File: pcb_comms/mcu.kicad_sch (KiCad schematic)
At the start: 25 parts, among them U2 STM32WLE5CCU6, Y1 G43270018, Y3 32MHz

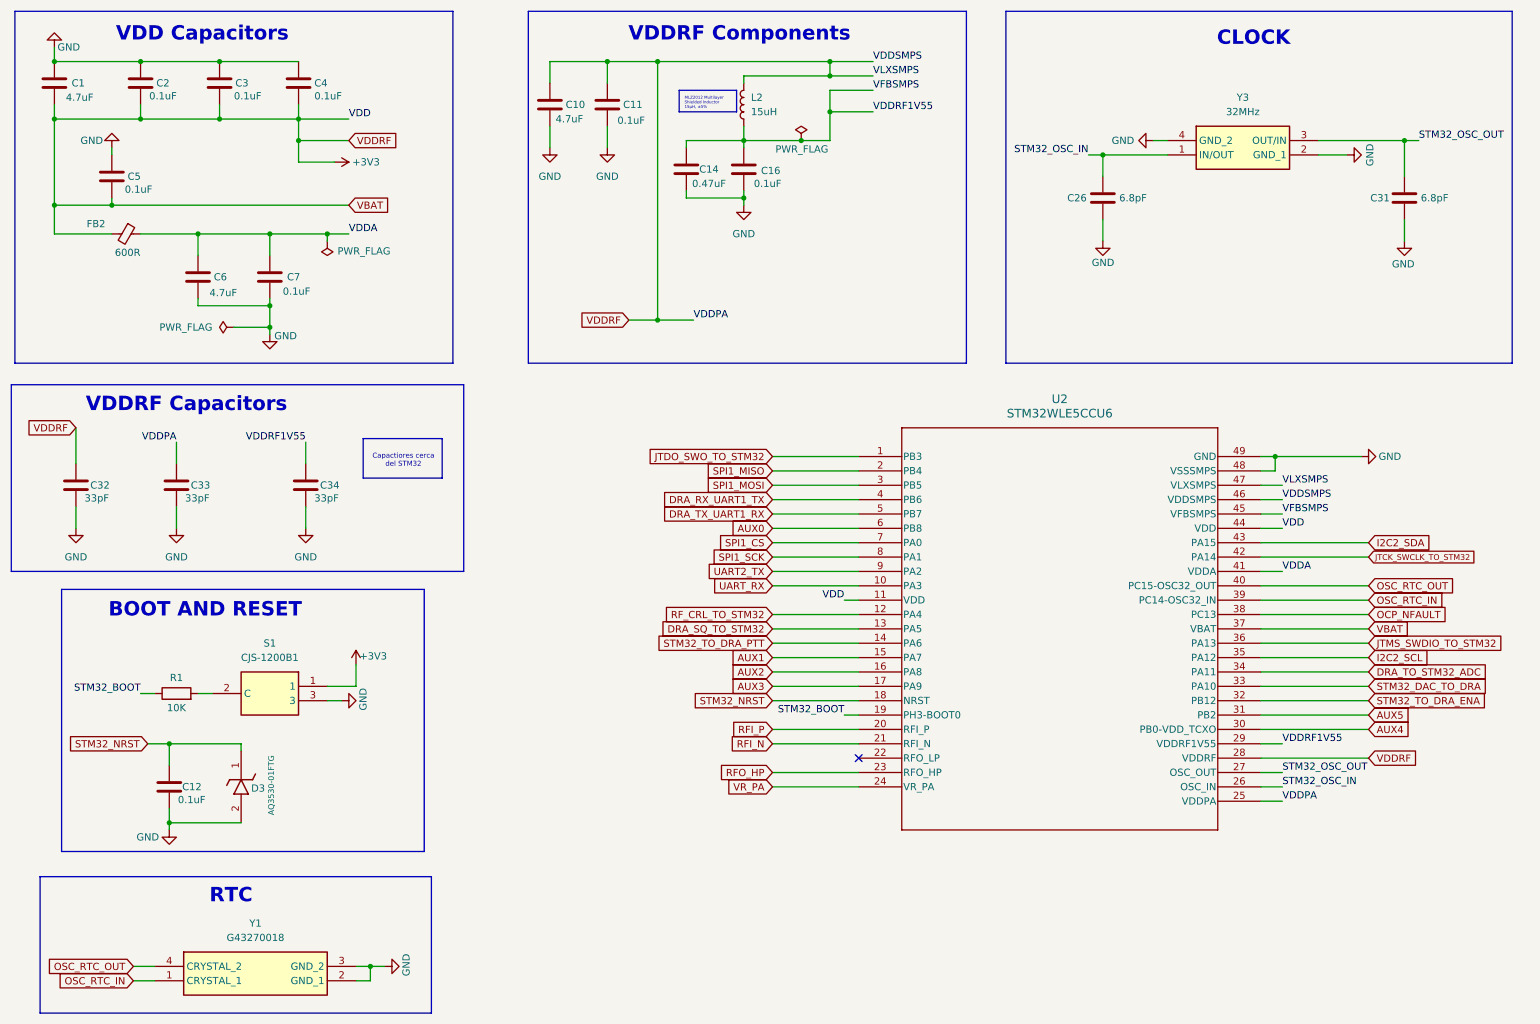
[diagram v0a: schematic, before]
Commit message: Route pcb
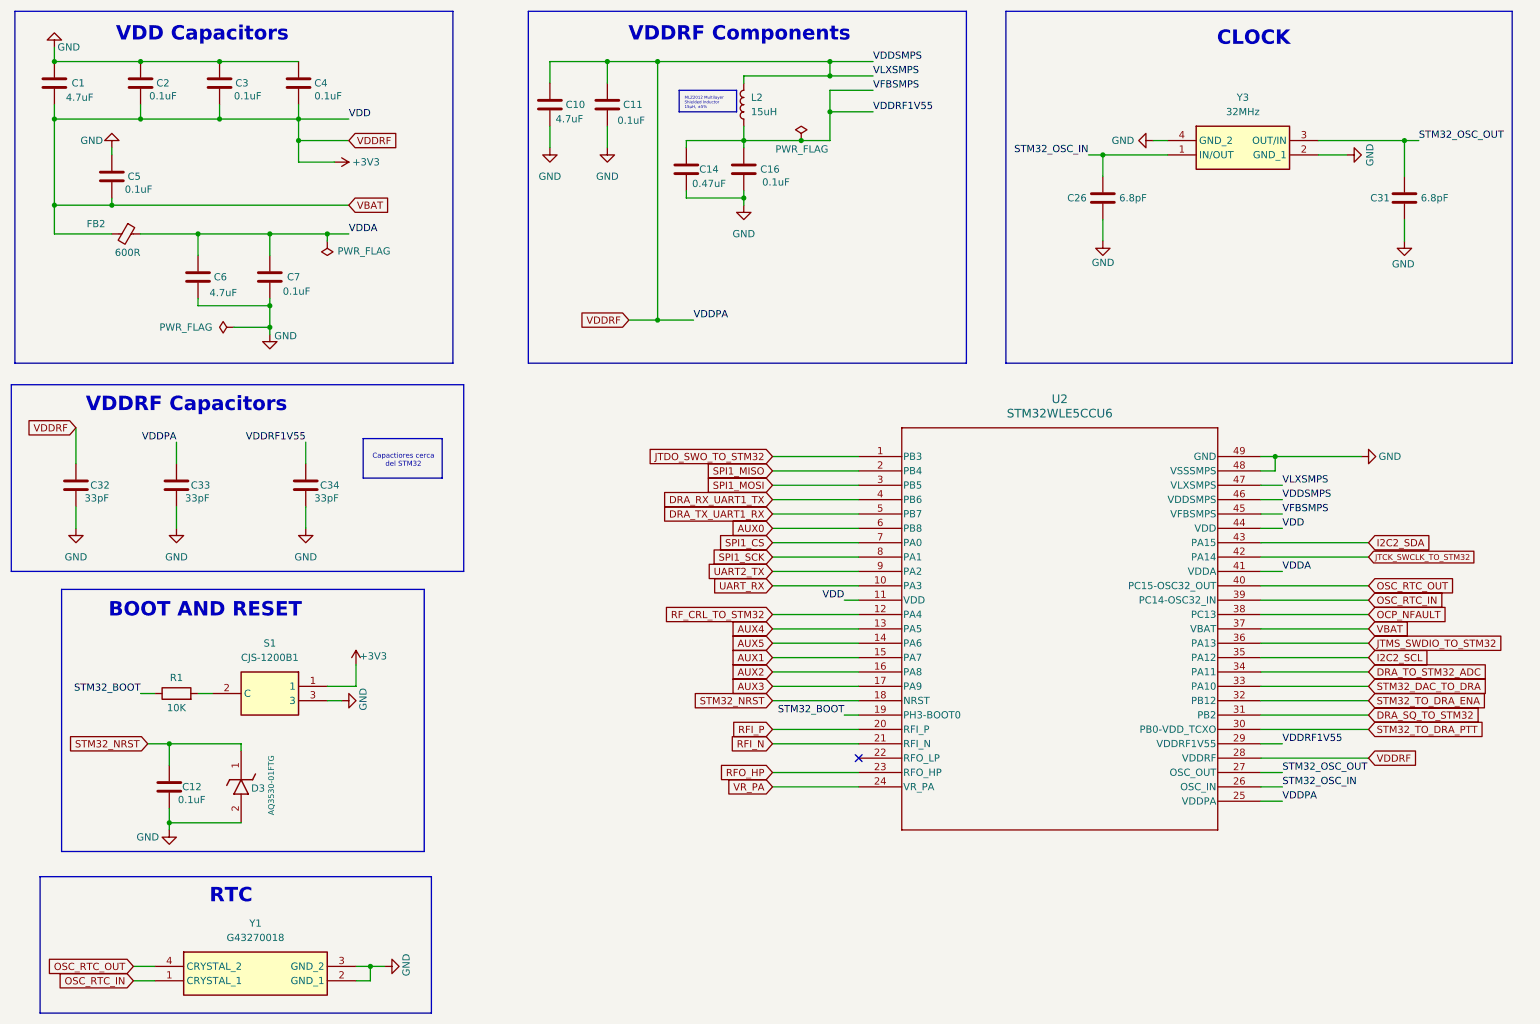
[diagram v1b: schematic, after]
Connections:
- net AUX4: now also U2.13 (PA5); no longer U2.30 (PB0-VDD_TCXO)
- net AUX5: now also U2.14 (PA6); no longer U2.31 (PB2)
- net DRA_SQ_TO_STM32: now also U2.31 (PB2); no longer U2.13 (PA5)
- net STM32_TO_DRA_PTT: now also U2.30 (PB0-VDD_TCXO); no longer U2.14 (PA6)
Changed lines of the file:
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@@
 	(wire
 		(pts
+			(xy 152.4 129.54) (xy 167.64 129.54)
+		)
+		(stroke
+			(width 0)
+			(type default)
+		)
+	)
+	(wire
+		(pts
 			(xy 147.32 40.64) (xy 147.32 41.91)
 		)
@@
 	(wire
 		(pts
-			(xy 152.4 127) (xy 167.64 127)
-		)
-		(stroke
-			(width 0)
-			(type default)
-		)
-	)
-	(wire
-		(pts
 			(xy 241.3 99.06) (xy 241.3 96.52)
 		)
@@
 	(wire
 		(pts
+			(xy 152.4 127) (xy 167.64 127)
+		)
+		(stroke
+			(width 0)
+			(type default)
+		)
+	)
+	(wire
+		(pts
 			(xy 152.4 134.62) (xy 167.64 134.62)
 		)
@@
 	(wire
 		(pts
-			(xy 238.76 142.24) (xy 257.81 142.24)
-		)
-		(stroke
-			(width 0)
-			(type default)
-		)
-	)
-	(wire
-		(pts
 			(xy 25.4 57.15) (xy 35.56 57.15)
 		)
@@
 	(wire
 		(pts
-			(xy 238.76 144.78) (xy 257.81 144.78)
-		)
-		(stroke
-			(width 0)
-			(type default)
-		)
-	)
-	(wire
-		(pts
 			(xy 45.72 147.32) (xy 58.42 147.32)
 		)
@@
 	(wire
 		(pts
+			(xy 238.76 142.24) (xy 257.81 142.24)
+		)
+		(stroke
+			(width 0)
+			(type default)
+		)
+	)
+	(wire
+		(pts
 			(xy 165.1 121.92) (xy 167.64 121.92)
 		)
@@
 	(wire
 		(pts
-			(xy 39.37 186.69) (xy 43.18 186.69)
+			(xy 238.76 144.78) (xy 257.81 144.78)
 		)
 		(stroke
@@
 	(wire
 		(pts
-			(xy 77.47 40.64) (xy 68.58 40.64)
+			(xy 39.37 186.69) (xy 43.18 186.69)
 		)
 		(stroke
@@
 	(wire
 		(pts
-			(xy 73.66 57.15) (xy 73.66 58.42)
+			(xy 77.47 40.64) (xy 68.58 40.64)
 		)
 		(stroke
@@
 	(wire
 		(pts
-			(xy 113.03 26.67) (xy 113.03 30.48)
+			(xy 73.66 57.15) (xy 73.66 58.42)
 		)
 		(stroke
@@
 	(wire
 		(pts
-			(xy 152.4 139.7) (xy 167.64 139.7)
+			(xy 113.03 26.67) (xy 113.03 30.48)
 		)
 		(stroke
@@
 	(wire
 		(pts
-			(xy 78.74 137.16) (xy 78.74 133.35)
+			(xy 152.4 139.7) (xy 167.64 139.7)
 		)
 		(stroke
@@
 	(wire
 		(pts
-			(xy 152.4 129.54) (xy 167.64 129.54)
+			(xy 78.74 137.16) (xy 78.74 133.35)
 		)
 		(stroke
@@
 	(global_label "DRA_SQ_TO_STM32"
 		(shape input)
-		(at 152.4 127 180)
+		(at 257.81 142.24 0)
 		(effects
 			(font
 				(size 1.27 1.27)
 			)
-			(justify right)
+			(justify left)
 		)
 		(property "Intersheetrefs" "${INTERSHEET_REFS}"
-			(at 130.7278 114.3 0)
+			(at 279.4822 129.54 0)
 			(effects
 				(font
 					(size 1.27 1.27)
 				)
-				(justify right)
+				(justify left)
 				(hide yes)
 			)
@@
 	(global_label "STM32_TO_DRA_PTT"
 		(shape input)
-		(at 152.4 129.54 180)
+		(at 257.81 144.78 0)
 		(fields_autoplaced yes)
 		(effects
@@
 				(size 1.27 1.27)
 			)
-			(justify right)
+			(justify left)
 		)
 		(property "Intersheetrefs" "${INTERSHEET_REFS}"
-			(at 131.3326 129.54 0)
+			(at 278.8774 144.78 0)
 			(effects
 				(font
 					(size 1.27 1.27)
 				)
-				(justify right)
+				(justify left)
 				(hide yes)
 			)
@@
 	(global_label "AUX4"
 		(shape input)
-		(at 257.81 144.78 0)
+		(at 152.4 127 180)
 		(fields_autoplaced yes)
 		(effects
@@
 				(size 1.27 1.27)
 			)
-			(justify left)
+			(justify right)
 		)
 		(property "Intersheetrefs" "${INTERSHEET_REFS}"
-			(at 265.6333 144.78 0)
+			(at 144.5767 127 0)
 			(effects
 				(font
 					(size 1.27 1.27)
 				)
-				(justify left)
+				(justify right)
 				(hide yes)
 			)
@@
 	(global_label "AUX5"
 		(shape input)
-		(at 257.81 142.24 0)
+		(at 152.4 129.54 180)
 		(fields_autoplaced yes)
 		(effects
@@
 				(size 1.27 1.27)
 			)
-			(justify left)
+			(justify right)
 		)
 		(property "Intersheetrefs" "${INTERSHEET_REFS}"
-			(at 265.6333 142.24 0)
+			(at 144.5767 129.54 0)
 			(effects
 				(font
 					(size 1.27 1.27)
 				)
-				(justify left)
+				(justify right)
 				(hide yes)
 			)
@@
 		(lib_id "Device:C")
 		(at 147.32 45.72 0)
+		(mirror y)
 		(unit 1)
 		(exclude_from_sim no)
@@
 		(dnp no)
 		(property "Reference" "C16"
-			(at 150.368 45.974 0)
+			(at 153.67 45.72 0)
 			(effects
 				(font
@@
 		)
 		(property "Value" "0.1uF"
-			(at 149.098 48.26 0)
+			(at 155.448 48.006 0)
 			(effects
 				(font
@@
 		)
 		(property "Footprint" "Capacitor_SMD:C_0805_2012Metric_Pad1.18x1.45mm_HandSolder"
-			(at 148.2852 49.53 0)
+			(at 146.3548 49.53 0)
 			(effects
 				(font
@@
 		(on_board yes)
 		(dnp no)
-		(fields_autoplaced yes)
 		(property "Reference" "L2"
 			(at 148.59 33.0199 0)

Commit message: Update route
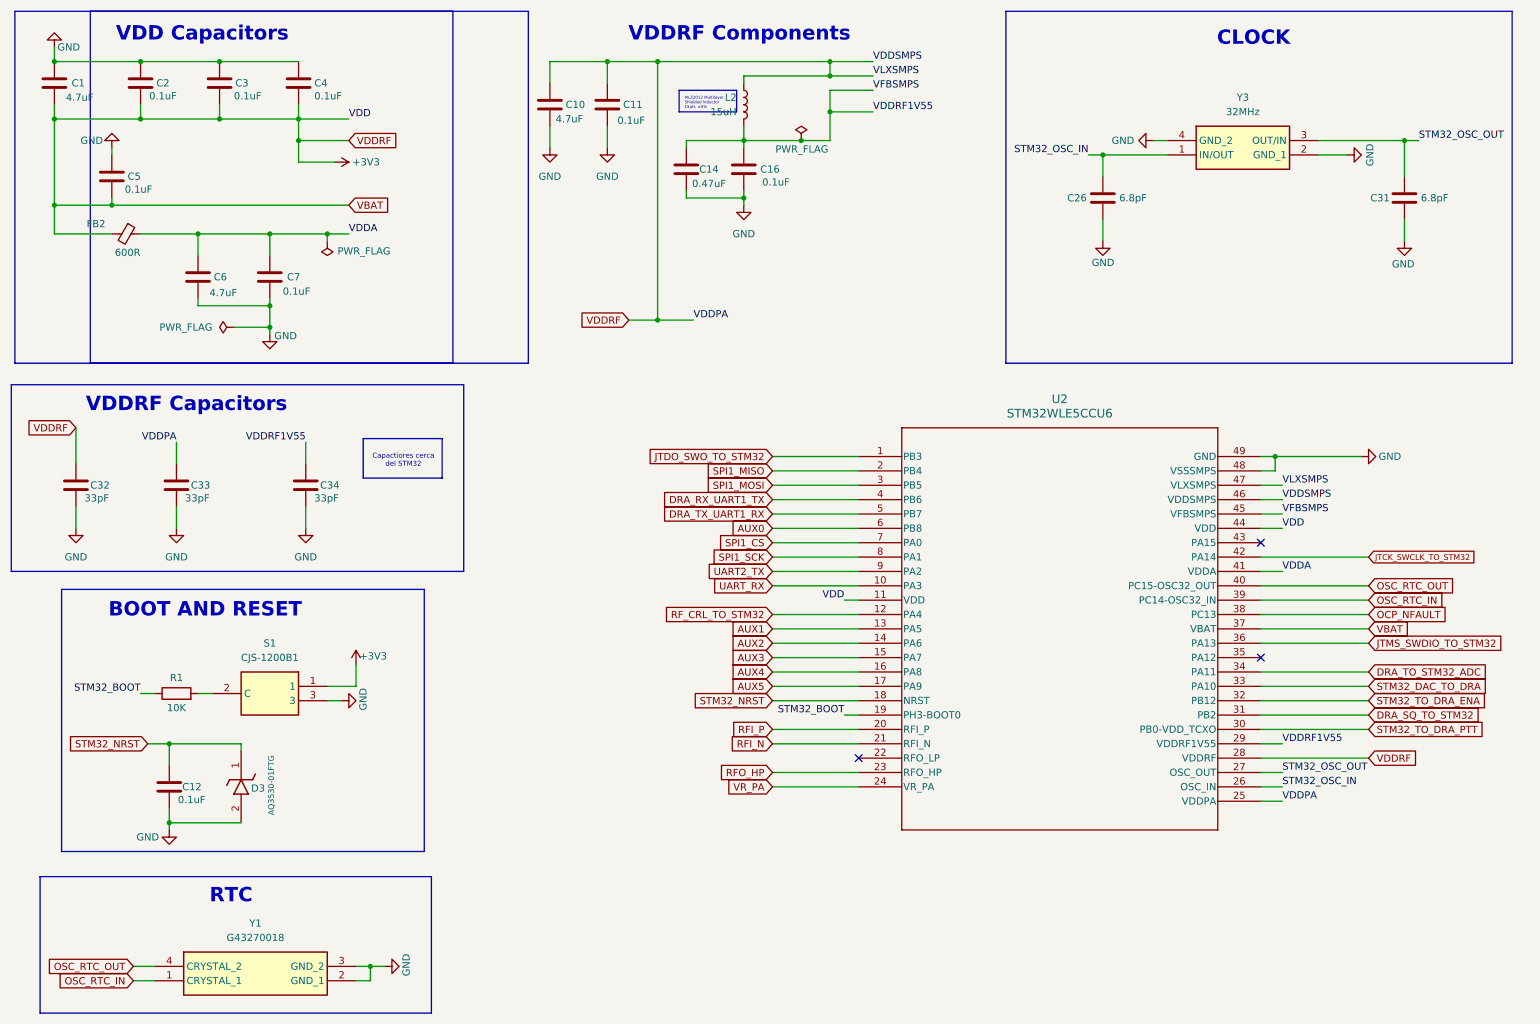
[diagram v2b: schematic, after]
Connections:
- net AUX1: now also U2.13 (PA5); no longer U2.15 (PA7)
- net AUX2: now also U2.14 (PA6); no longer U2.16 (PA8)
- net AUX3: now also U2.15 (PA7); no longer U2.17 (PA9)
- net AUX4: now also U2.16 (PA8); no longer U2.13 (PA5)
- net AUX5: now also U2.17 (PA9); no longer U2.14 (PA6)
- net I2C2_SCL: no longer names the net of U2.35 (PA12)
- net I2C2_SDA: no longer names the net of U2.43 (PA15)
- no-connect marks 1 -> 3
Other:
- moved on the sheet: L2
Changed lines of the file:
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@@
 		(exclude_from_sim no)
 		(at 109.22 17.78 0)
-		(size 77.47 62.23)
+		(size -77.47 62.23)
 		(margins 0.9525 0.9525 0.9525 0.9525)
 		(stroke
@@
 				(size 1.27 1.27)
 			)
-			(justify left top)
+			(justify right top)
 		)
 	)
@@
 	)
 	(no_connect
+		(at 238.76 111.76)
+	)
+	(no_connect
 		(at 167.64 149.86)
 	)
+	(no_connect
+		(at 238.76 132.08)
+	)
 	(wire
 		(pts
@@
 	(wire
 		(pts
-			(xy 152.4 129.54) (xy 167.64 129.54)
-		)
-		(stroke
-			(width 0)
-			(type default)
-		)
-	)
-	(wire
-		(pts
 			(xy 147.32 40.64) (xy 147.32 41.91)
 		)
@@
 	(wire
 		(pts
-			(xy 238.76 111.76) (xy 257.81 111.76)
+			(xy 152.4 144.78) (xy 167.64 144.78)
 		)
 		(stroke
@@
 	(wire
 		(pts
-			(xy 152.4 144.78) (xy 167.64 144.78)
+			(xy 241.3 99.06) (xy 241.3 96.52)
 		)
 		(stroke
@@
 	(wire
 		(pts
-			(xy 241.3 99.06) (xy 241.3 96.52)
+			(xy 210.82 54.61) (xy 210.82 58.42)
 		)
 		(stroke
@@
 	(wire
 		(pts
-			(xy 210.82 54.61) (xy 210.82 58.42)
+			(xy 29.21 105.41) (xy 29.21 109.22)
 		)
 		(stroke
@@
 	(wire
 		(pts
-			(xy 29.21 105.41) (xy 29.21 109.22)
+			(xy 152.4 137.16) (xy 167.64 137.16)
 		)
 		(stroke
@@
 	(wire
 		(pts
-			(xy 238.76 132.08) (xy 257.81 132.08)
-		)
-		(stroke
-			(width 0)
-			(type default)
-		)
-	)
-	(wire
-		(pts
 			(xy 147.32 38.1) (xy 147.32 40.64)
 		)
@@
 	(wire
 		(pts
-			(xy 152.4 127) (xy 167.64 127)
-		)
-		(stroke
-			(width 0)
-			(type default)
-		)
-	)
-	(wire
-		(pts
-			(xy 152.4 134.62) (xy 167.64 134.62)
-		)
-		(stroke
-			(width 0)
-			(type default)
-		)
-	)
-	(wire
-		(pts
 			(xy 248.92 43.18) (xy 254 43.18)
 		)
@@
 	(wire
 		(pts
-			(xy 25.4 57.15) (xy 35.56 57.15)
+			(xy 152.4 127) (xy 167.64 127)
 		)
 		(stroke
@@
 	(wire
 		(pts
-			(xy 238.76 121.92) (xy 257.81 121.92)
+			(xy 25.4 57.15) (xy 35.56 57.15)
 		)
 		(stroke
@@
 	(wire
 		(pts
-			(xy 152.4 132.08) (xy 167.64 132.08)
+			(xy 238.76 121.92) (xy 257.81 121.92)
 		)
 		(stroke
@@
 	(wire
 		(pts
-			(xy 152.4 137.16) (xy 167.64 137.16)
-		)
-		(stroke
-			(width 0)
-			(type default)
-		)
-	)
-	(wire
-		(pts
 			(xy 152.4 104.14) (xy 167.64 104.14)
 		)
@@
 	(wire
 		(pts
+			(xy 152.4 132.08) (xy 167.64 132.08)
+		)
+		(stroke
+			(width 0)
+			(type default)
+		)
+	)
+	(wire
+		(pts
 			(xy 242.57 101.6) (xy 238.76 101.6)
 		)
@@
 	(wire
 		(pts
+			(xy 152.4 134.62) (xy 167.64 134.62)
+		)
+		(stroke
+			(width 0)
+			(type default)
+		)
+	)
+	(wire
+		(pts
 			(xy 170.18 29.21) (xy 162.56 29.21)
 		)
@@
 	(wire
 		(pts
+			(xy 152.4 129.54) (xy 167.64 129.54)
+		)
+		(stroke
+			(width 0)
+			(type default)
+		)
+	)
+	(wire
+		(pts
 			(xy 152.4 111.76) (xy 167.64 111.76)
 		)
@@
 		)
 	)
-	(global_label "I2C2_SDA"
-		(shape input)
-		(at 257.81 111.76 0)
-		(fields_autoplaced yes)
-		(effects
-			(font
-				(size 1.27 1.27)
-			)
-			(justify left)
-		)
-		(property "Intersheetrefs" "${INTERSHEET_REFS}"
-			(at 269.6247 111.76 0)
-			(effects
-				(font
-					(size 1.27 1.27)
-				)
-				(justify left)
-				(hide yes)
-			)
-		)
-	)
 	(global_label "DRA_SQ_TO_STM32"
 		(shape input)
@@
 	(global_label "AUX3"
 		(shape input)
-		(at 152.4 137.16 180)
+		(at 152.4 132.08 180)
 		(fields_autoplaced yes)
 		(effects
@@
 		)
 		(property "Intersheetrefs" "${INTERSHEET_REFS}"
-			(at 144.5767 137.16 0)
+			(at 144.5767 132.08 0)
 			(effects
 				(font
@@
 	(global_label "AUX4"
 		(shape input)
-		(at 152.4 127 180)
+		(at 152.4 134.62 180)
 		(fields_autoplaced yes)
 		(effects
@@
 		)
 		(property "Intersheetrefs" "${INTERSHEET_REFS}"
-			(at 144.5767 127 0)
+			(at 144.5767 134.62 0)
 			(effects
 				(font
@@
 	(global_label "AUX2"
 		(shape input)
-		(at 152.4 134.62 180)
+		(at 152.4 129.54 180)
 		(fields_autoplaced yes)
 		(effects
@@
 		)
 		(property "Intersheetrefs" "${INTERSHEET_REFS}"
-			(at 144.5767 134.62 0)
+			(at 144.5767 129.54 0)
 			(effects
 				(font
@@
 		)
 	)
-	(global_label "I2C2_SCL"
-		(shape input)
-		(at 257.81 132.08 0)
-		(fields_autoplaced yes)
-		(effects
-			(font
-				(size 1.27 1.27)
-			)
-			(justify left)
-		)
-		(property "Intersheetrefs" "${INTERSHEET_REFS}"
-			(at 269.5642 132.08 0)
-			(effects
-				(font
-					(size 1.27 1.27)
-				)
-				(justify left)
-				(hide yes)
-			)
-		)
-	)
 	(global_label "AUX1"
 		(shape input)
-		(at 152.4 132.08 180)
+		(at 152.4 127 180)
 		(fields_autoplaced yes)
 		(effects
@@
 		)
 		(property "Intersheetrefs" "${INTERSHEET_REFS}"
-			(at 144.5767 132.08 0)
+			(at 144.5767 127 0)
 			(effects
 				(font
@@
 	(global_label "AUX5"
 		(shape input)
-		(at 152.4 129.54 180)
+		(at 152.4 137.16 180)
 		(fields_autoplaced yes)
 		(effects
@@
 		)
 		(property "Intersheetrefs" "${INTERSHEET_REFS}"
-			(at 144.5767 129.54 0)
+			(at 144.5767 137.16 0)
 			(effects
 				(font
@@
 		(lib_id "Device:L")
 		(at 147.32 34.29 0)
-		(mirror y)
 		(unit 1)
 		(exclude_from_sim no)
@@
 		(dnp no)
 		(property "Reference" "L2"
-			(at 148.59 33.0199 0)
+			(at 146.05 33.0199 0)
 			(effects
 				(font
@@
 		)
 		(property "Value" "15uH"
-			(at 148.59 35.5599 0)
+			(at 146.05 35.5599 0)
 			(effects
 				(font
